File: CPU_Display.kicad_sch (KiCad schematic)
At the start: 3 parts

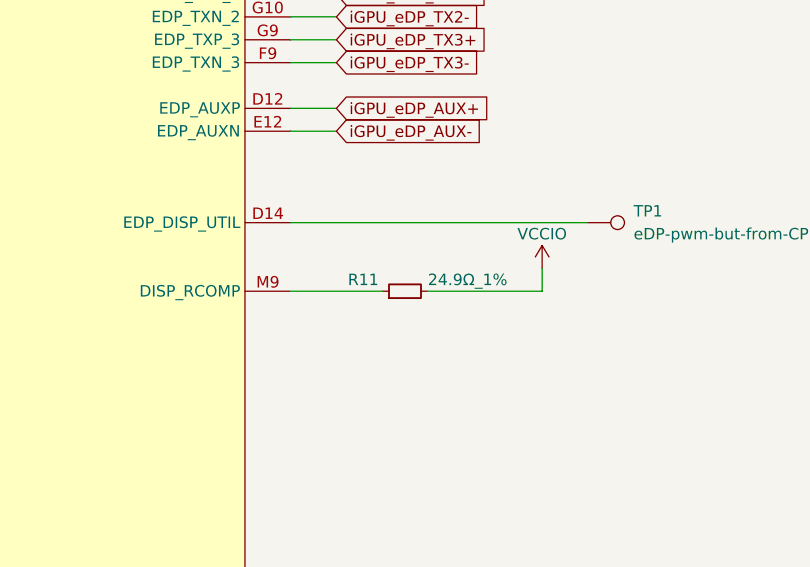
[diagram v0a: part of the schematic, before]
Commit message: implemented some misc cpu signals
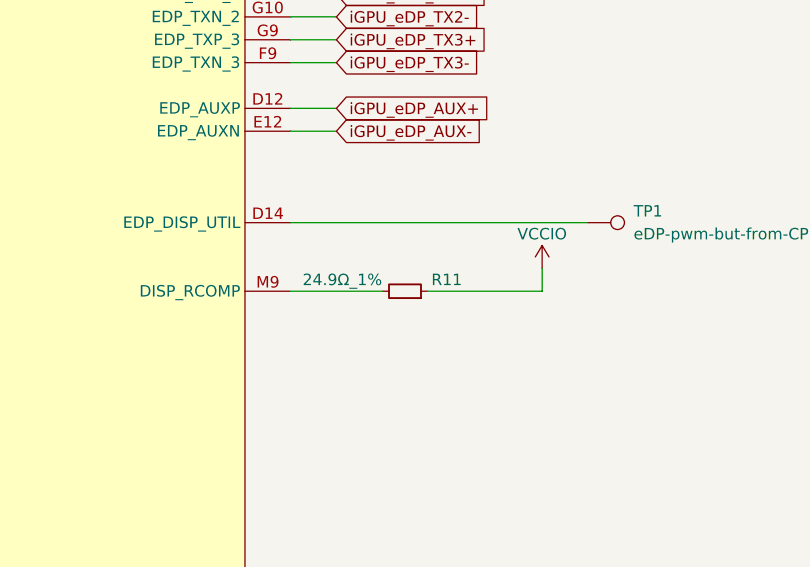
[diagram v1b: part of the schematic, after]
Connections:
- net VCCIO: now also R11.1; no longer R11.2
- net at JCPU1.M9 (DISP_RCOMP): now also R11.2; no longer R11.1
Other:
- moved on the sheet: R11
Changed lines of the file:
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@@
 	(symbol
 		(lib_id "Device:R_Small")
-		(at 191.77 91.44 90)
+		(at 191.77 91.44 270)
+		(mirror x)
 		(unit 1)
 		(exclude_from_sim no)
@@
 		(dnp no)
 		(property "Reference" "R11"
-			(at 185.42 90.17 90)
+			(at 198.12 90.17 90)
 			(effects
 				(font
@@
 		)
 		(property "Value" "24.9Ω_1%"
-			(at 194.31 90.17 90)
+			(at 189.23 90.17 90)
 			(effects
 				(font
